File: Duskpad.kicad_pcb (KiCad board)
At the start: 2 copper layers, 82.5 x 100 mm, 54 parts, among them J1 OLED display, SW1 SW_Push, SW10 SW_Push, SW11 SW_Push, SW12 SW_Push, SW13 SW_Push, SW14 SW_Push, SW15 SW_Push, SW16 SW_Push, SW2 SW_Push, SW3 SW_Push, SW4 SW_Push, SW5 SW_Push, SW6 SW_Push, SW7 SW_Push, SW8 SW_Push, SW9 SW_Push, U1 MOUDLE-SEEEDUINO-XIAO

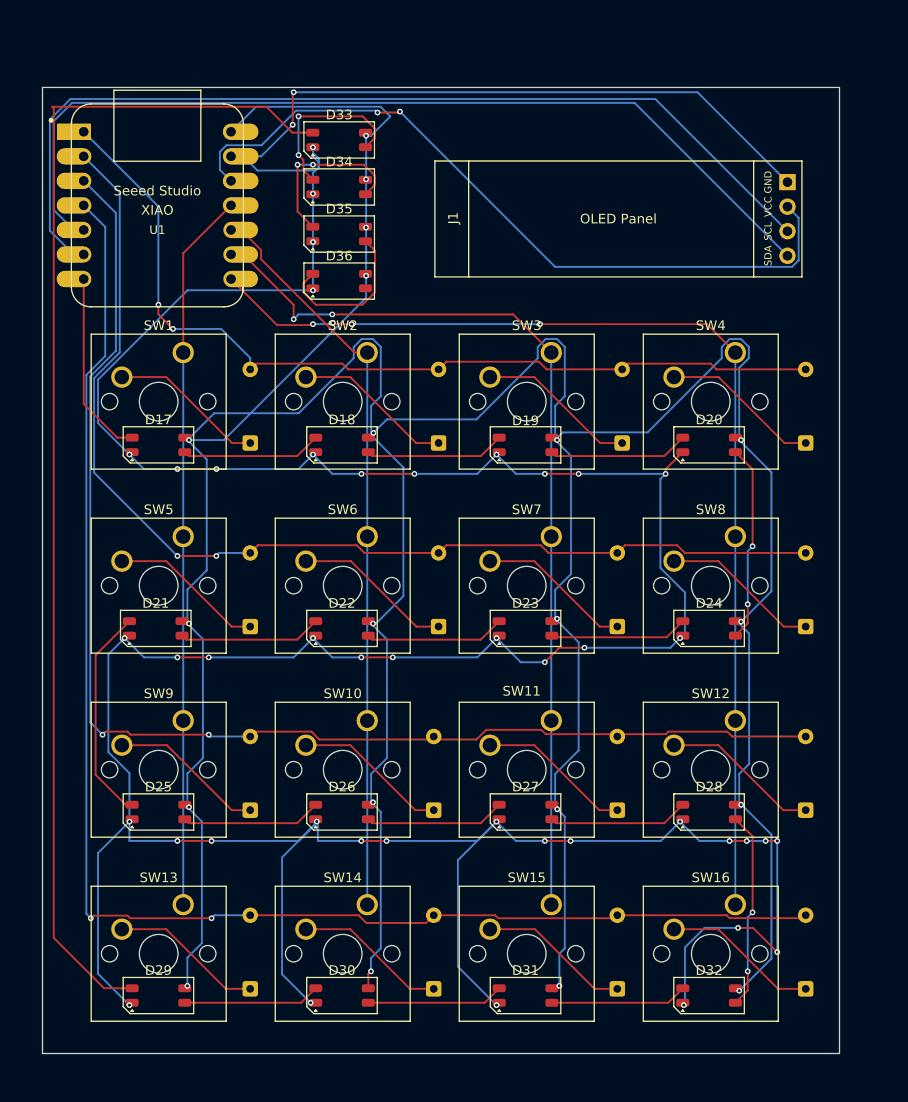
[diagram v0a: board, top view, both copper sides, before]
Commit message: updates
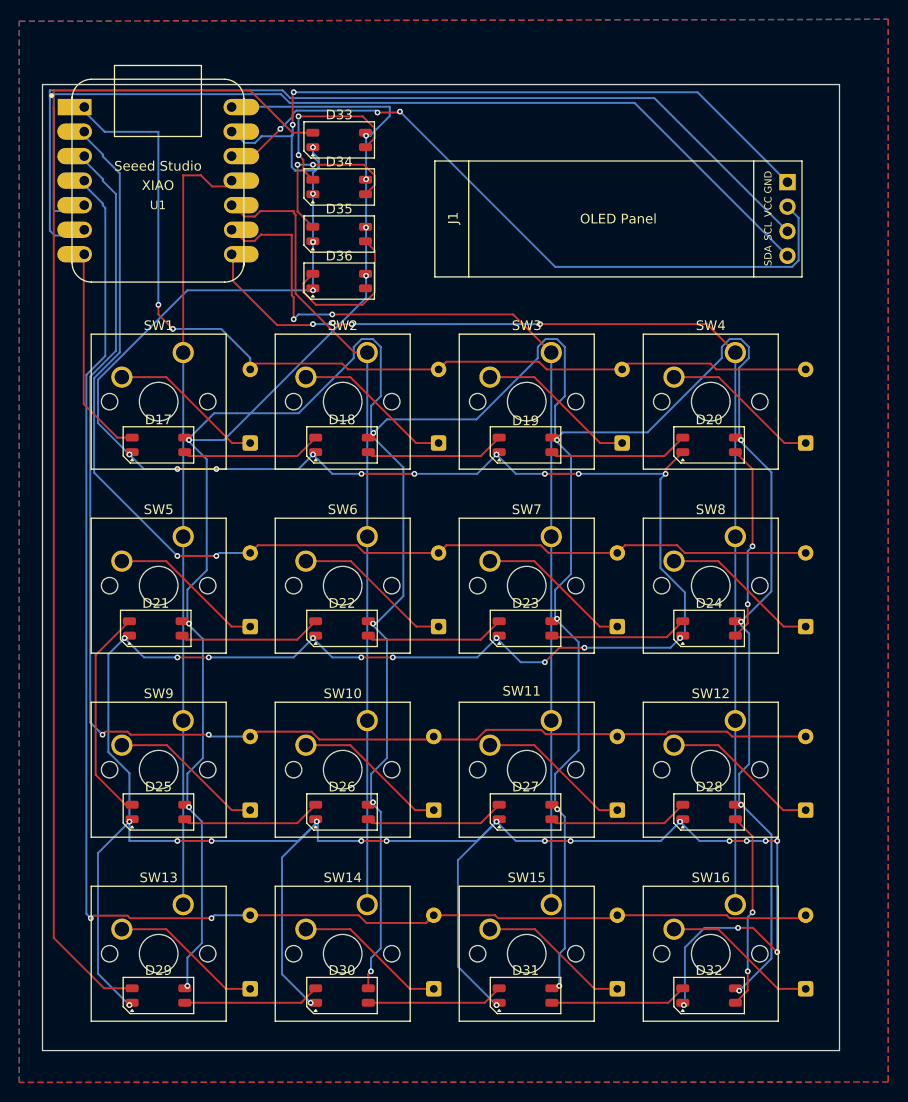
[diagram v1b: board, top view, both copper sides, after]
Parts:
- moved U1 2.56 mm to (80.6, 34.3)
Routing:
- net Colunm 1: track 74.9 -> 81.7 mm
- net Colunm 2: track 77.1 -> 82.9 mm
- net Row 1: track 93.8 -> 99.6 mm
- net Colunm 3: track 95.8 -> 101.5 mm
- net VCC(3V): track 78.3 -> 74.4 mm, vias 2 -> 3
- net GND: track 469.5 -> 466.6 mm
- net DIN: track 19.4 -> 22.0 mm
- net Row 4: track 151.2 -> 153.8 mm
- net Row 2: track 114.7 -> 117.3 mm
- net Row 3: track 134.9 -> 137.5 mm
- net Colunm 4: track 112.7 -> 115.2 mm
- net Net-(D29-DIN): track 124.5 -> 126.7 mm
- net Net-(J1-Pin_3): track 98.9 -> 101.0 mm
- net Net-(J1-Pin_4): track 96.4 -> 98.3 mm
- added copper zone on B.Cu, net (none)
- added copper zone on F.Cu, net (none)
